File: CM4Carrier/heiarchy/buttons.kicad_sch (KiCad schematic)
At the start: 7 parts, among them SW1 SW_Push, U2 74HC00

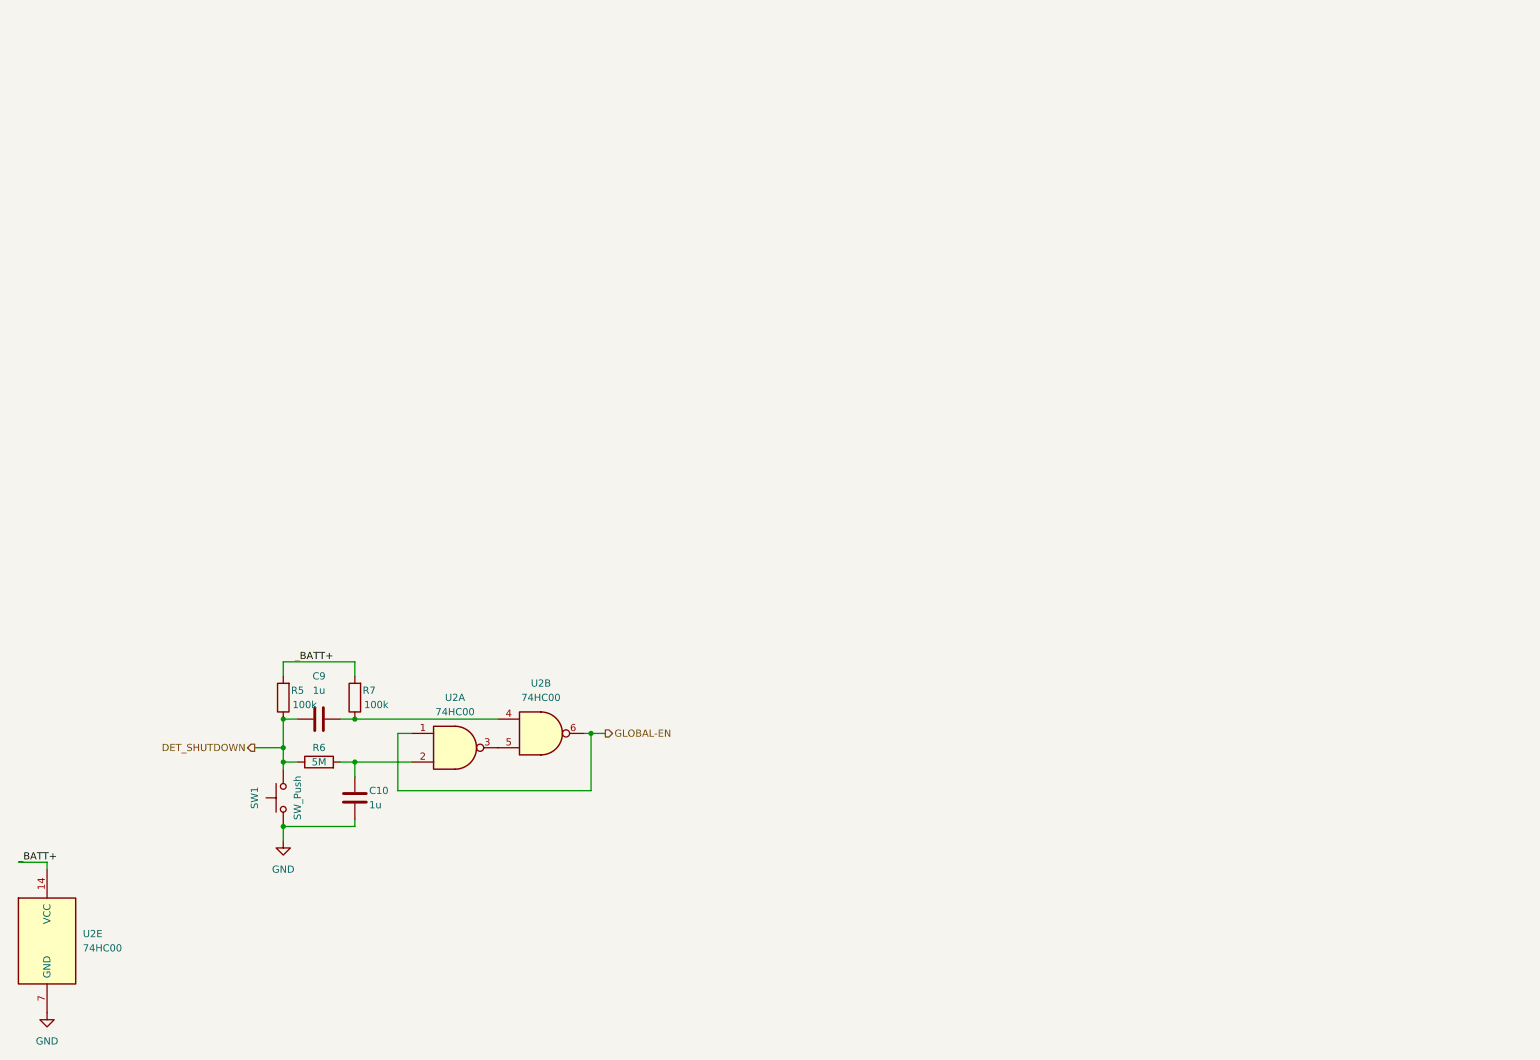
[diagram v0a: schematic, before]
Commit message: Additions
- Fixed gitignore (Backups)
- Work on buttons
- Work on ADC for JOYSTICK
- Work on some other stuff
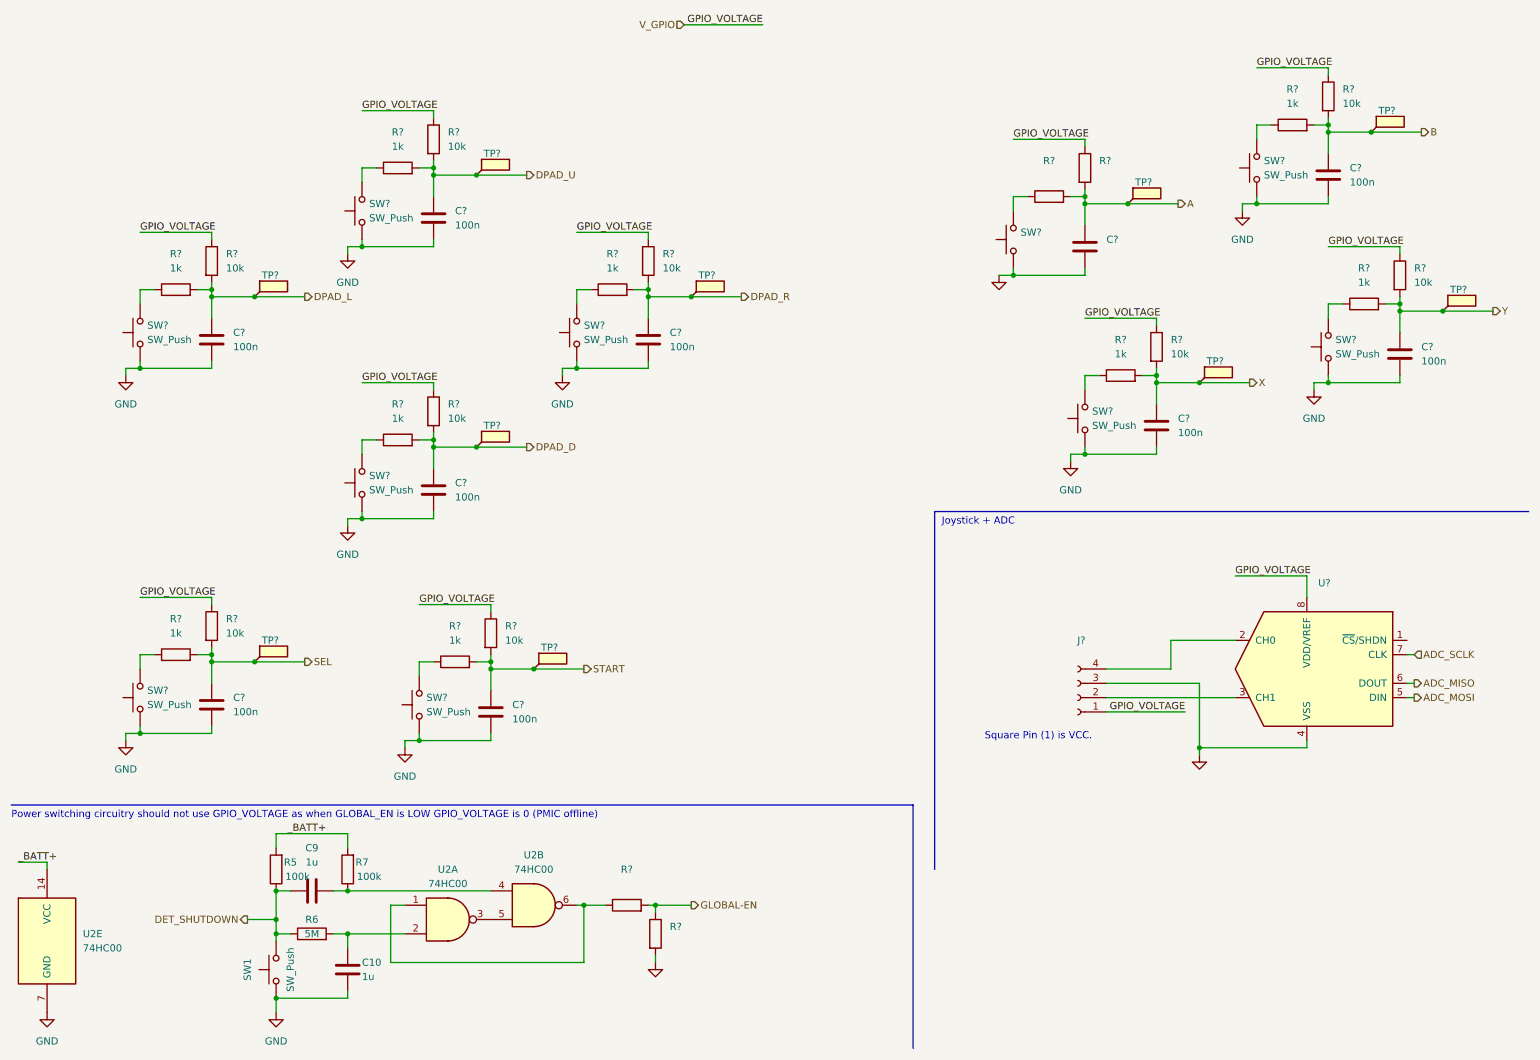
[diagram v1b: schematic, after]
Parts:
- added C?: (no value), symbol Device:C
- added C? (x9): 100n, symbol Device:C
- added J?: (no value), symbol Connector:Conn_01x04_Female
- added R? (x4): (no value), symbol Device:R
- added R? (x9): 1k, symbol Device:R
- added R? (x9): 10k, symbol Device:R
- added SW?: (no value), symbol Switch:SW_Push
- added SW? (x9): SW_Push, symbol Switch:SW_Push
- added TP? (x9): ~, symbol Connector:TestPoint_Flag
- added TP?: (no value), symbol Connector:TestPoint_Flag
- added U?: (no value), symbol Analog_ADC:MCP3002
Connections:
- net GLOBAL-EN: now also R?.1, R?.2; no longer U2.1, U2.6
- net GND: now also C?.2, C?.2, C?.2, C?.2, C?.2, C?.2, C?.2, C?.2, C?.2, C?.2, J?.3 (Pin_3), R?.2, SW?.1, SW?.1, SW?.1, SW?.1, SW?.1, SW?.1, SW?.1, SW?.1, SW?.1, SW?.1, U?.4 (VSS)
- new net: R?.1, SW?.2 (x10)
- new net: R?.1, U2.1, U2.6
- new net: J?.4 (Pin_4), U?.2 (CH0)
- new net: J?.2 (Pin_2), U?.3 (CH1)
- new net A: C?.1, R?.2, R?.2, TP?.1
- new net ADC_MISO: U?.6 (DOUT)
- new net ADC_MOSI: U?.5 (DIN)
- new net ADC_SCLK: U?.7 (CLK)
- new net B: C?.1, R?.2, R?.2, TP?.1
- new net DPAD_D: C?.1, R?.2, R?.2, TP?.1
- new net DPAD_L: C?.1, R?.2, R?.2, TP?.1
- new net DPAD_R: C?.1, R?.2, R?.2, TP?.1
- new net DPAD_U: C?.1, R?.2, R?.2, TP?.1
- new net SEL: C?.1, R?.2, R?.2, TP?.1
- new net START: C?.1, R?.2, R?.2, TP?.1
- new net V_GPIO: J?.1 (Pin_1), R?.1, R?.1, R?.1, R?.1, R?.1, R?.1, R?.1, R?.1, R?.1, R?.1, U?.8 (VDD/VREF)
- new net X: C?.1, R?.2, R?.2, TP?.1
- new net Y: C?.1, R?.2, R?.2, TP?.1
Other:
- note added: "Joystick + ADC"
- note added: "Power switching circuitry should not use GPIO_VOLTAGE as when GLOBAL_EN is LOW GPIO_VOLTAGE is 0 (PMIC offline)"
- note added: "Square Pin (1) is VCC."
- moved on the sheet: C10, C9, R5, R6, R7, SW1, U2A, U2B
